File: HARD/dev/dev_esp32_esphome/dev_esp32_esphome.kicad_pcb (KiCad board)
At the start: 2 copper layers, 69 parts, among them J1 USB4105-GF-A, Q1 DMG3415U, SW1 SW_Push, SW2 SW_Push, U1 SHTC3, U2 ICM-42670-P, U3 ESP32-C3-MINI-1, U4 MCP73831T-2ACI/OT, U5 ESP_ASSISTANT, U6 SY8088, U7 BME280, Y1 32.768Hz

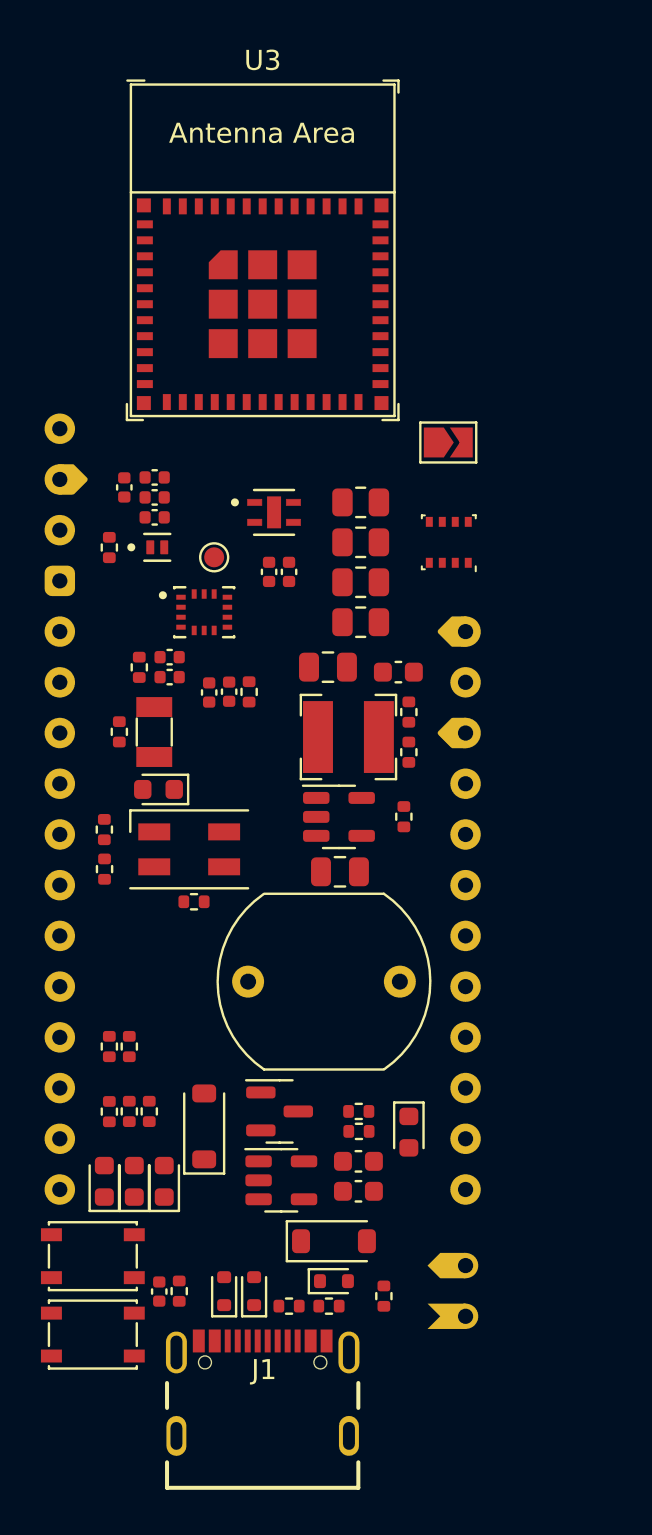
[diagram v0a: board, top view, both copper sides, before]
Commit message: With route
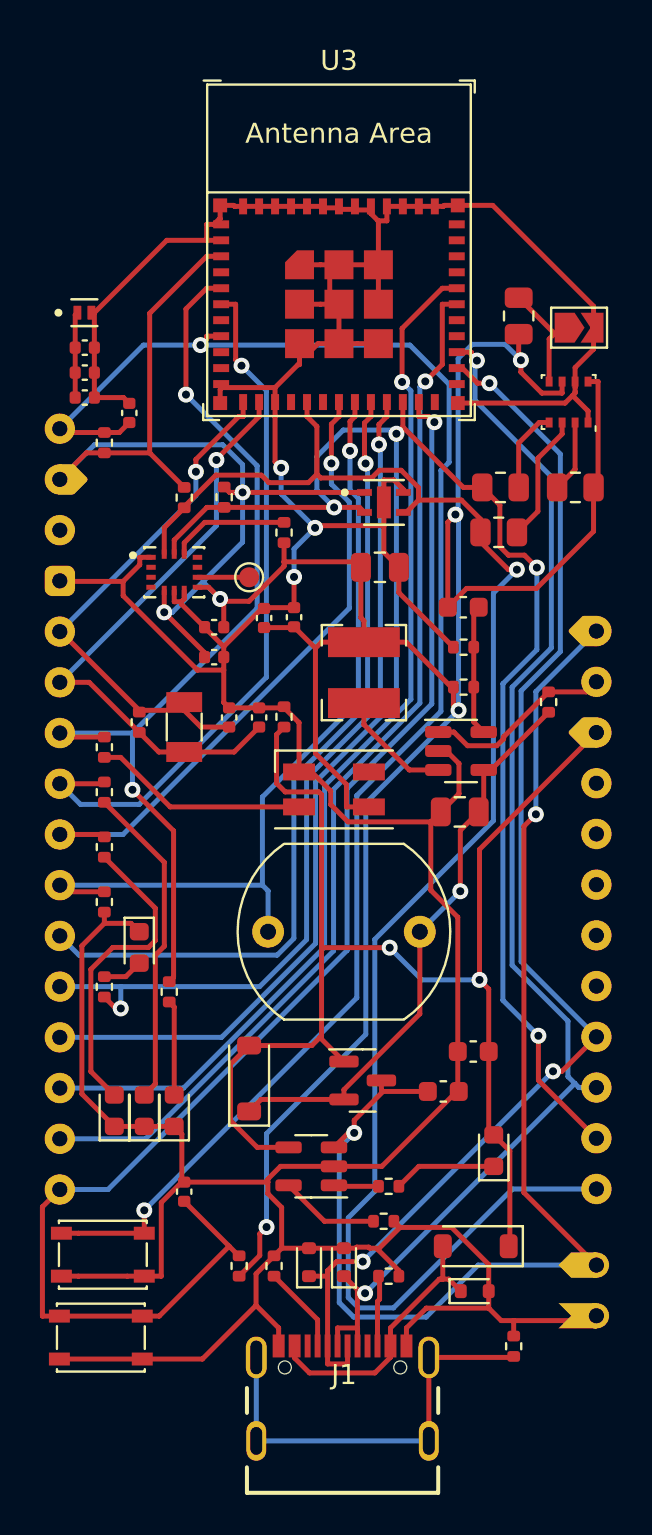
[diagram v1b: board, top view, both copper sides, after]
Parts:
- moved R14 28.1 mm to (104.8, 49.7), turned to -90 degrees
- moved R15 27.6 mm to (102.8, 49.8), turned to -90 degrees
- moved R21 17.3 mm to (119.5, 40.7), turned to -90 degrees
- moved R23 16.0 mm to (98.8, 64.5)
- moved R24 13.3 mm to (98.8, 67.3)
- moved D1 12.3 mm to (97.8, 40.5)
- moved R20 11.8 mm to (122.3, 49.2), turned to 180 degrees
- moved R1 9.91 mm to (107.8, 51.5)
- moved R10 9.25 mm to (121.0, 60.0)
- moved U7 9.24 mm to (122.0, 45.0)
- moved R25 8.96 mm to (114.5, 71.5), turned to 180 degrees
- moved JP1 8.72 mm to (122.5, 41.2)
- moved D2 7.97 mm to (100.5, 72.3), turned to -90 degrees
- moved C12 7.96 mm to (117.2, 77.5)
- moved D3 7.85 mm to (110.2, 64.4)
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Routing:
- net GND: track 0.00 -> 255.4 mm, vias 0 -> 3
- net +3V3: track 0.00 -> 174.4 mm, vias 0 -> 7
- net IO8_SCL: track 0.00 -> 104.3 mm, vias 0 -> 4
- net IO10_SDA: track 0.00 -> 83.7 mm, vias 0 -> 1
- net CHIP_PU: track 0.00 -> 80.1 mm, vias 0 -> 2
- net IO9_BOOT: track 0.00 -> 70.6 mm, vias 0 -> 1
- net VBUS: track 0.00 -> 68.1 mm, vias 0 -> 2
- net +BATT: track 0.00 -> 64.6 mm, vias 0 -> 2
- net USB_D-: track 0.00 -> 64.3 mm, vias 0 -> 3
- net USB_D+: track 0.00 -> 63.3 mm, vias 0 -> 2
- net IO20_RX: track 0.00 -> 53.0 mm, vias 0 -> 1
- net IO21_TX: track 0.00 -> 52.7 mm, vias 0 -> 1
- net IO2: track 0.00 -> 46.8 mm, vias 0 -> 2
- net IO7: track 0.00 -> 44.1 mm, vias 0 -> 2
- net IO5: track 0.00 -> 41.4 mm, vias 0 -> 1
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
